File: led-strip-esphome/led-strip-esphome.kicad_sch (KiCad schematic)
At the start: 4 parts, among them U1 TP4056_C725790

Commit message: pcb
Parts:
- removed TH1: Thermistor_NTC, symbol Device:Thermistor_NTC
- added C1, C2: 10uF, symbol Device:C
- added C3: RVT1E221M0607_C2918361, easyeda2kicad:CAP-SMD_BD6.3-L6.6-W6.6-LS7.4-FD, symbol easyeda2kicad:RVT1E221M0607_C2918361
- added C4, C5, C6, C7, C8: 22uF, symbol Device:C
- added D2, D3: LED, LED_SMD:LED_0603_1608Metric, symbol Device:LED
- added D4: D, symbol Device:D
- added D5: 1N5824_C7503125, easyeda2kicad:DO-27_BD5.3-L8.4-P12.40-D1.3-RD, symbol easyeda2kicad:1N5824_C7503125
- added L1: 33uh, symbol Device:L
- added L2: 3.3uh, symbol Device:L
- added R1: 2.4k, symbol Device:R
- added R2, R3: 210, symbol Device:R
- added R4: 0.4, symbol Device:R
- added R5: 1M, LED_SMD:LED_0805_2012Metric, symbol Device:R
- added R6, R7: 5.11k, symbol Device:R
- added R8: 33k, symbol Device:R
- added R9: 100k, symbol Device:R
- added U2: LM2596S-3.3, Package_TO_SOT_SMD:TO-263-5_TabPin3, symbol Regulator_Switching:LM2596S-3.3
- added U3: RVT1E681M1010_C5221838, easyeda2kicad:CAP-SMD_BD10.0-L10.3-W10.3-LS11.6-FD, symbol easyeda2kicad:RVT1E681M1010_C5221838
- added U4: AP2007SPER, easyeda2kicad:ESOP-8_L4.9-W3.9-P1.27-LS6.0-BL-EP, symbol easyeda2kicad:AP2007SPER
- added USB1: TYPE-C 6P(073), easyeda2kicad:TYPE-C-SMD_TYPE-C-6P_5, symbol easyeda2kicad:TYPE-C6P(073)
- D1: LCSC (none) -> C7423443
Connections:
- net at BT1.1 (+), U1.5 (BAT): now also C1.1
- net GND: now reaches BT1.2 (-)
- net GND: now also U1.1 (TEMP), U1.3 (GND), U1.4 (VCC), U1.8 (CE), C1.2, C2.1, C2.2, C3.2, C4.2, C5.2, C6.2, C7.2, C8.2, D2.2 (A), D3.2 (A), D5.2 (A), R1.2, R4.2, R5.2, R6.2, R7.2, R8.2, U2.3 (GND), U2.5 (~{ON}/OFF), U3.2, U4.5 (GND), USB1.A12 (GND), USB1.B12 (GND)
- net at U1.2 (PROG): now also R1.1
- net at U1.6 (~{STDBY}): now also R3.2
- net at U1.7 (~{CHRG}): now also R2.2
- new net: R5.1, USB1.7 (EH)
- new net: R6.1, USB1.A5 (CC1)
- new net: D4.2 (A), USB1.A9 (VBUS), USB1.B9 (VBUS)
- new net: R7.1, USB1.B5 (CC2)
- new net: C6.1, C7.1, C8.1, R9.1, U2.1 (VIN), U3.1, U4.7 (VOUT), U4.8 (VOUT)
- new net: R8.1, R9.2
- new net: D5.1 (K), L1.1, U2.2 (OUT)
- new net: C3.1, L1.2, U2.4 (FB)
- new net: D3.1 (K), R2.1
- new net: C4.1, C5.1
- new net: L2.2, U4.1 (LX), U4.2 (LX)
- new net: L2.1, U4.3 (VIN), U4.4 (EN)
- new net: D2.1 (K), R3.1
- new net 3V~4.2V Out: D4.1 (K), R4.1
- no-connect marks 0 -> 1
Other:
- moved on the sheet: BT1, D1, U1

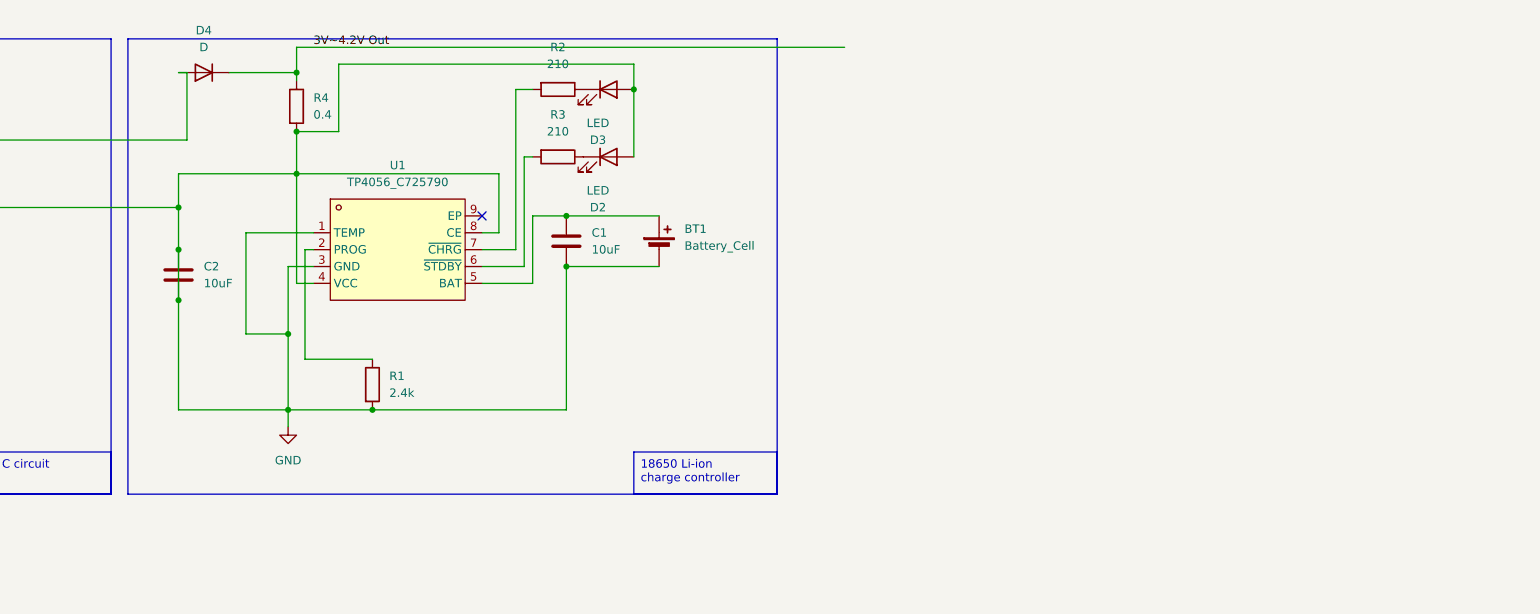
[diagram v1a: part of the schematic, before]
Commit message: pcb
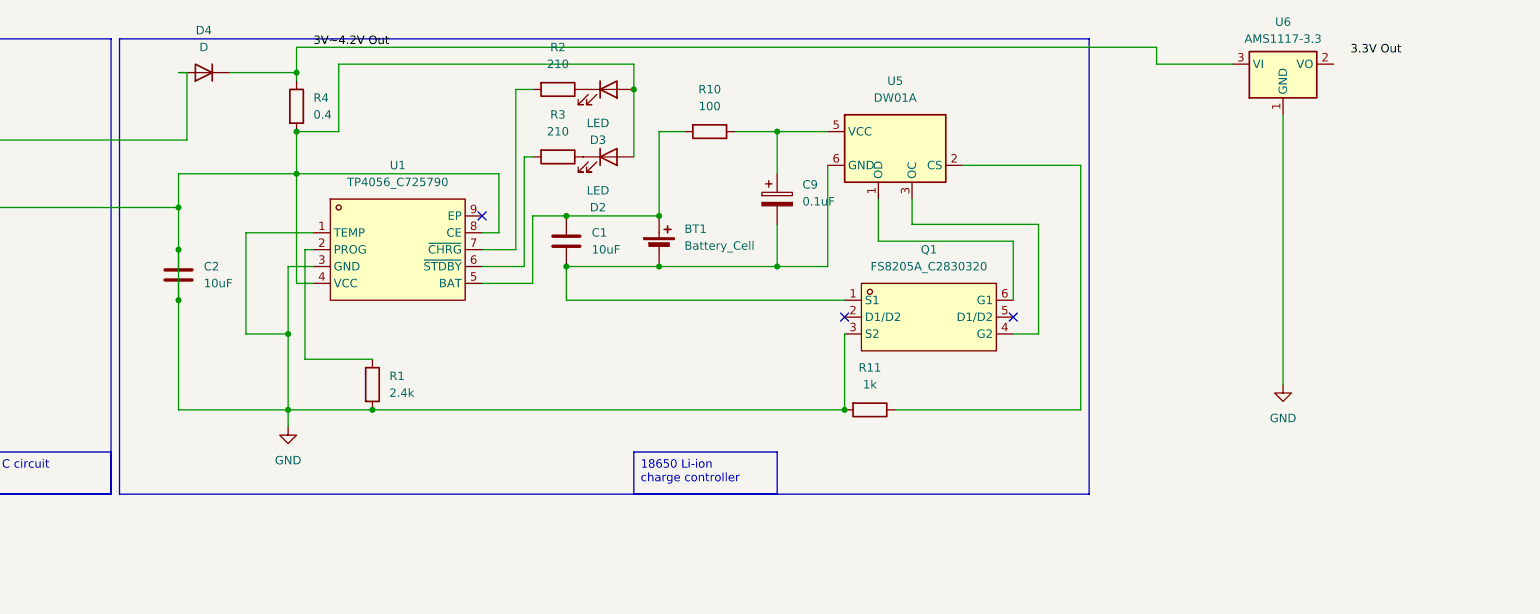
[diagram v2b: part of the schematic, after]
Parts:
- added C9: 0.1uF, Capacitor_SMD:CP_Elec_4x5.4, symbol Device:C_Polarized
- added Q1: FS8205A_C2830320, easyeda2kicad:SOT-23-6_L2.9-W1.6-P0.95-LS2.8-BR, symbol easyeda2kicad:FS8205A_C2830320
- added R10: 100, symbol Device:R
- added R11: 1k, symbol Device:R
- added U5: DW01A, Package_TO_SOT_SMD:SOT-23-6, symbol Battery_Management:DW01A
- added U6: AMS1117-3.3, Package_TO_SOT_SMD:SOT-223-3_TabPin2, symbol Regulator_Linear:AMS1117-3.3
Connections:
- net 3V~4.2V Out: now also U6.3 (VI)
- net GND: now also Q1.3 (S2), R11.2, U6.1 (GND); no longer BT1.2 (-), C1.2
- net at BT1.1 (+), C1.1, U1.5 (BAT): now also R10.2
- new net: BT1.2 (-), C1.2, C9.2, Q1.1 (S1), U5.6 (GND)
- new net: C9.1, R10.1, U5.5 (VCC)
- new net: Q1.4 (G2), U5.3 (OC)
- new net: Q1.6 (G1), U5.1 (OD)
- new net: R11.1, U5.2 (CS)
- no-connect marks 1 -> 3

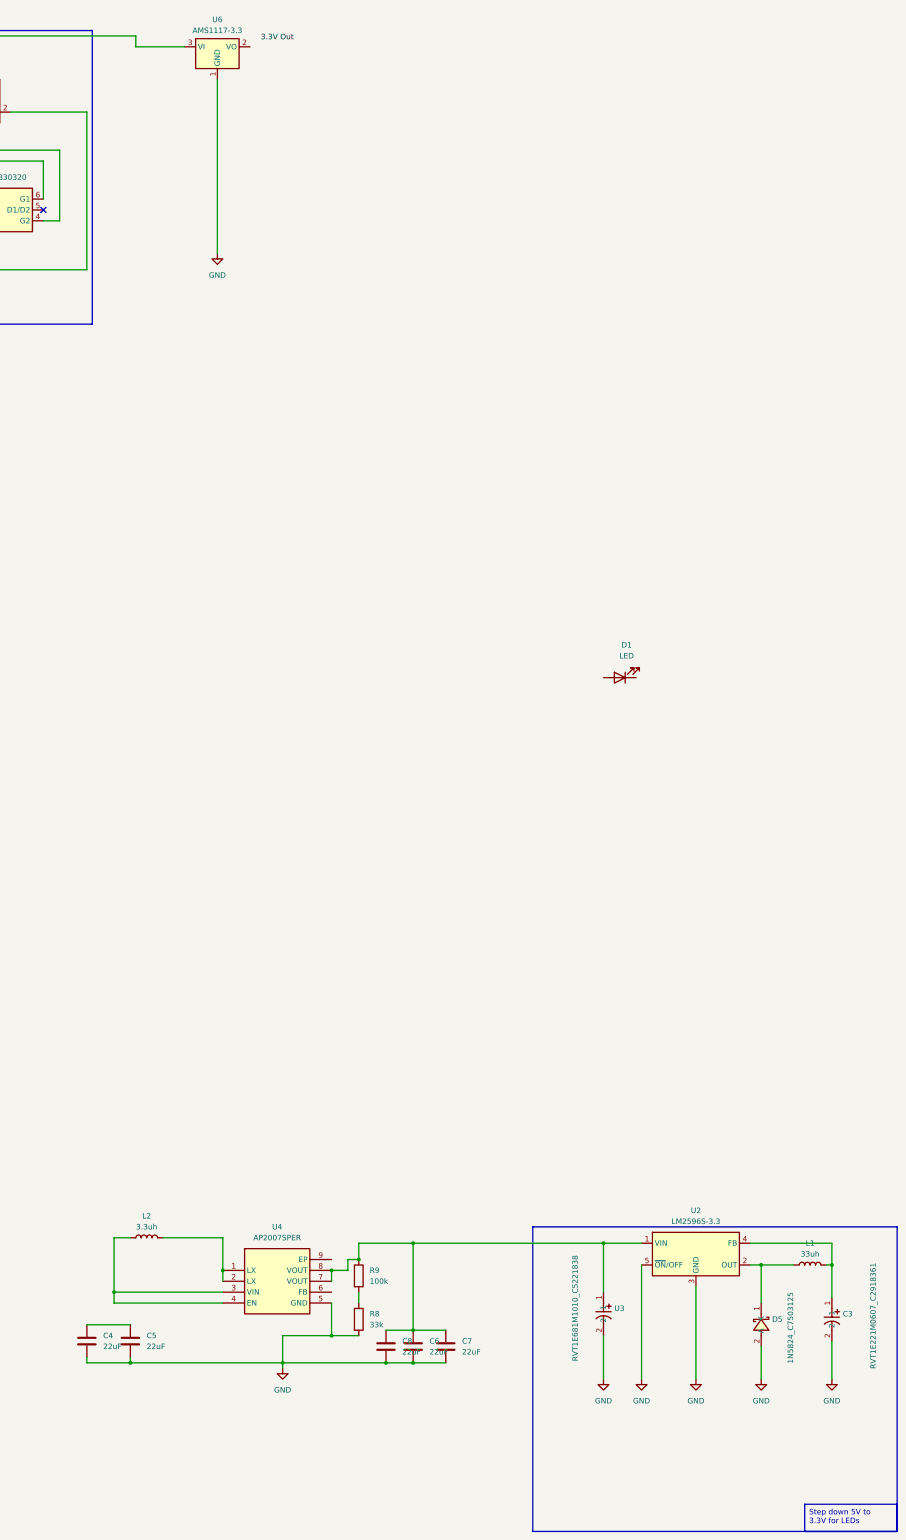
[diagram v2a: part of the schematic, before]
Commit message: pcb
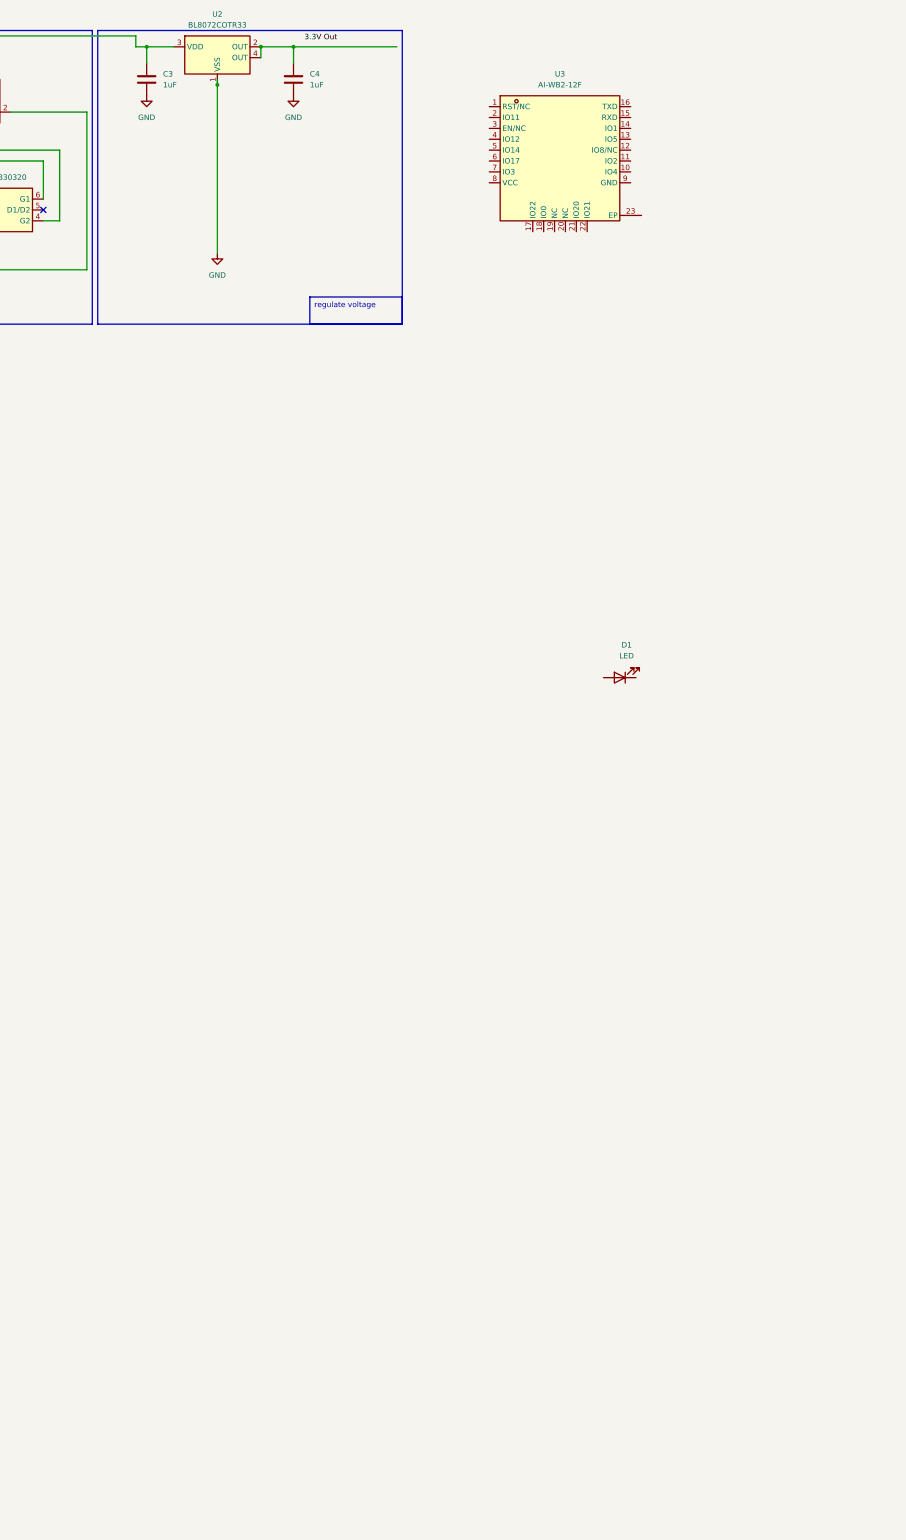
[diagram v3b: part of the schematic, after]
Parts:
- removed C3: RVT1E221M0607_C2918361, easyeda2kicad:CAP-SMD_BD6.3-L6.6-W6.6-LS7.4-FD, symbol easyeda2kicad:RVT1E221M0607_C2918361
- removed C5, C6, C7, C8: 22uF, symbol Device:C
- removed D5: 1N5824_C7503125, easyeda2kicad:DO-27_BD5.3-L8.4-P12.40-D1.3-RD, symbol easyeda2kicad:1N5824_C7503125
- removed L1: 33uh, symbol Device:L
- removed L2: 3.3uh, symbol Device:L
- removed R8: 33k, symbol Device:R
- removed R9: 100k, symbol Device:R
- removed U2: LM2596S-3.3, Package_TO_SOT_SMD:TO-263-5_TabPin3, symbol Regulator_Switching:LM2596S-3.3
- removed U3: RVT1E681M1010_C5221838, easyeda2kicad:CAP-SMD_BD10.0-L10.3-W10.3-LS11.6-FD, symbol easyeda2kicad:RVT1E681M1010_C5221838
- removed U4: AP2007SPER, easyeda2kicad:ESOP-8_L4.9-W3.9-P1.27-LS6.0-BL-EP, symbol easyeda2kicad:AP2007SPER
- removed U6: AMS1117-3.3, Package_TO_SOT_SMD:SOT-223-3_TabPin2, symbol Regulator_Linear:AMS1117-3.3
- added C3: 1uF, symbol Device:C
- added U2: BL8072COTR33, easyeda2kicad:TO-252-3_L6.6-W6.1-P2.28-LS10.1-BL, symbol easyeda2kicad:BL8072COTR33
- added U3: AI-WB2-12F, easyeda2kicad:COMM-SMD_22P-L24.0-W16.0-P2.00_ZIGBEE, symbol easyeda2kicad:AI-WB2-12F
- C4: value 22uF -> 1uF
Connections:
- net 3V~4.2V Out: now also C3.1, U2.3 (VDD)
- net GND: now also C3.2, U2.1 (VSS)
- net at C4.1: now also U2.2 (OUT), U2.4 (OUT)

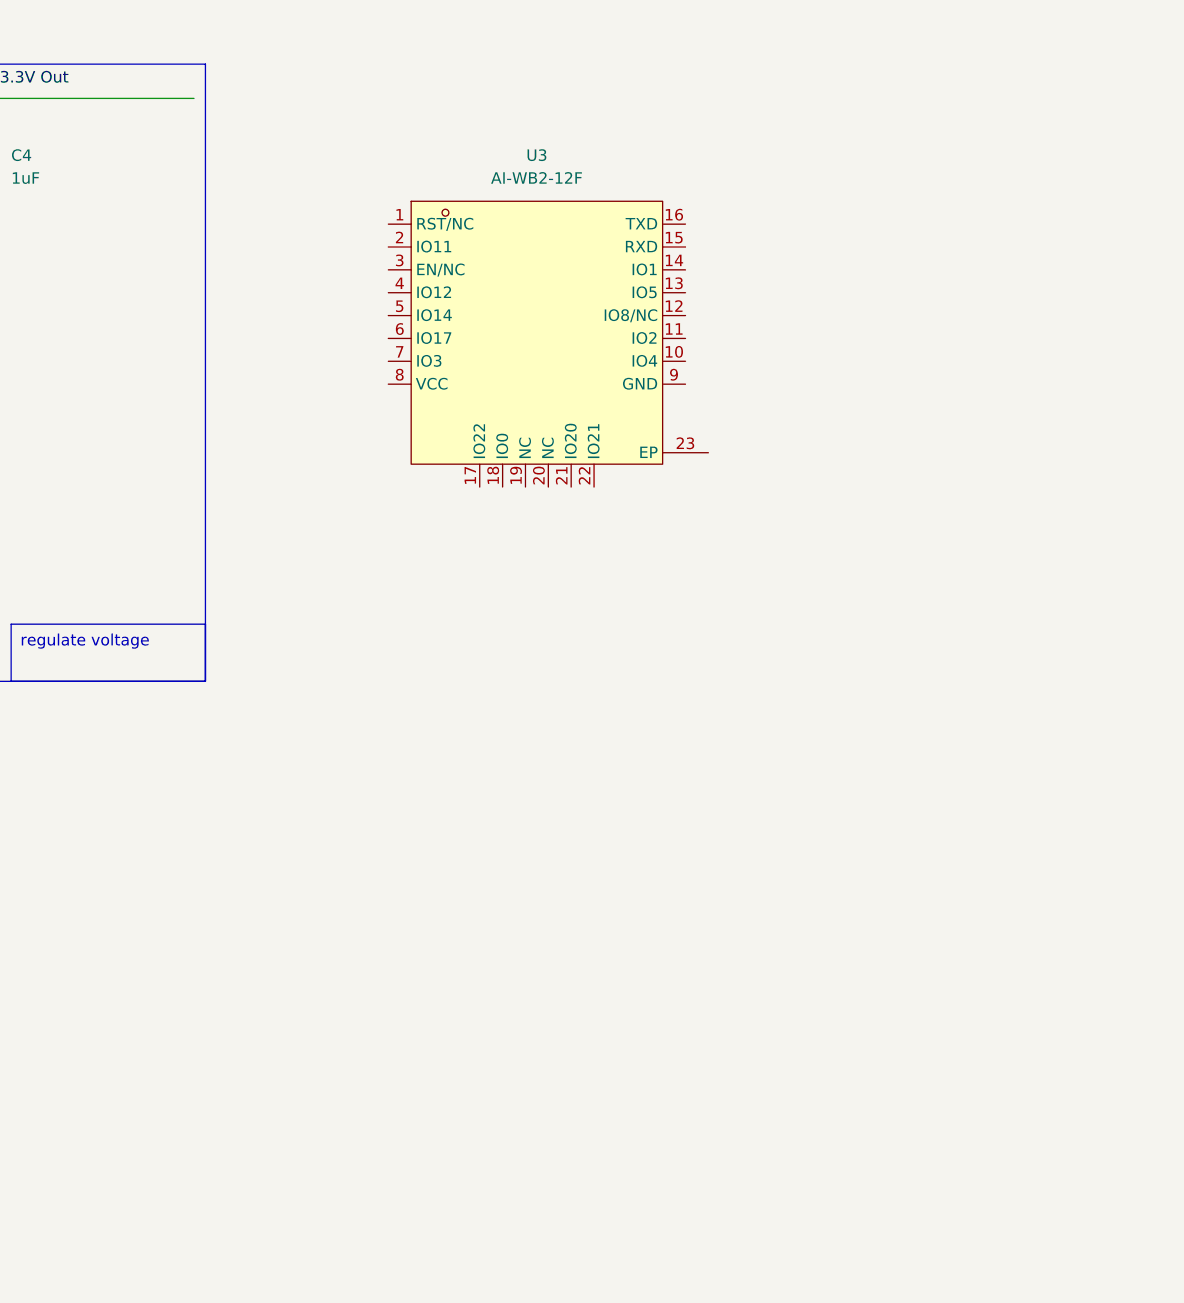
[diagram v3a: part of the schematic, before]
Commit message: pcb
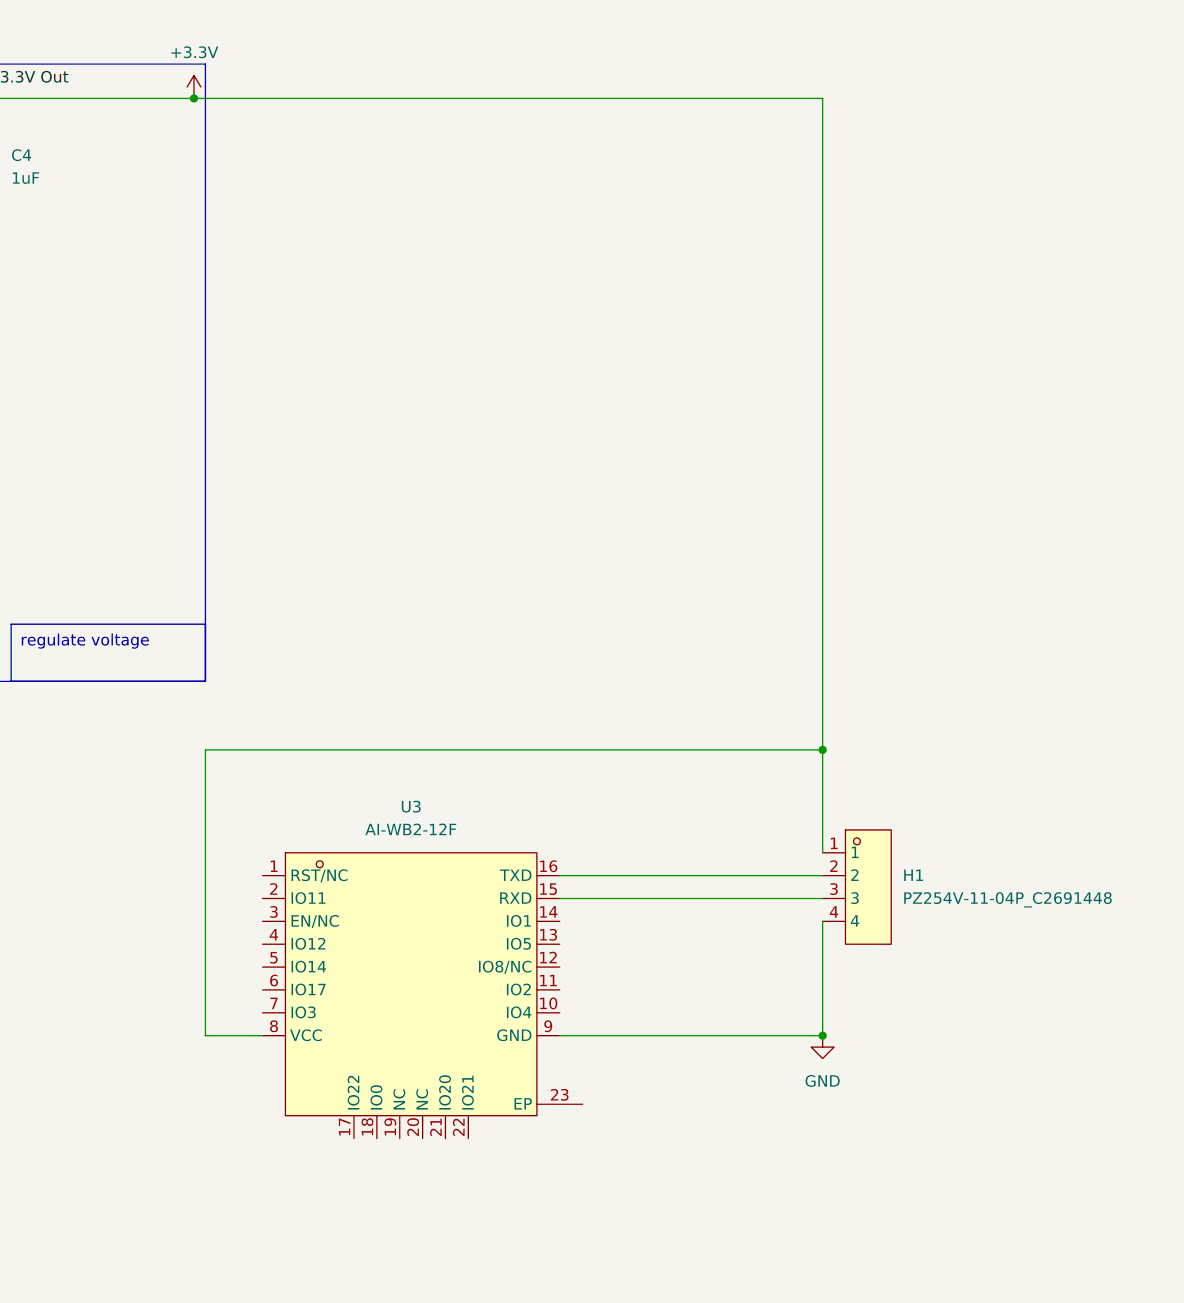
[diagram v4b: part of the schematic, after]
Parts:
- added H1: PZ254V-11-04P_C2691448, easyeda2kicad:HDR-TH_4P-P2.54-V-M, symbol easyeda2kicad:PZ254V-11-04P_C2691448
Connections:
- net GND: now also U3.9 (GND), H1.4
- net at U3.15 (RXD): now also H1.3
- net at U3.16 (TXD): now also H1.2
- net +3.3V: now reaches U3.8 (VCC)
- net +3.3V: now also C4.1, U2.2 (OUT), U2.4 (OUT), H1.1
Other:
- moved on the sheet: U3
